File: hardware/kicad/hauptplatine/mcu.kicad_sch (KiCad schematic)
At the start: 31 parts, among them J301 USB-C, J302 Debug (SWD + Serial1), SW301 Reset, SW302 BOOT, SW303 Service, SW304 Reedkontakt, U301 STM32F411CEU6, U302 USBLC6-2SC6, Y301 25MHz 12pF, Y302 32,768k 7pF

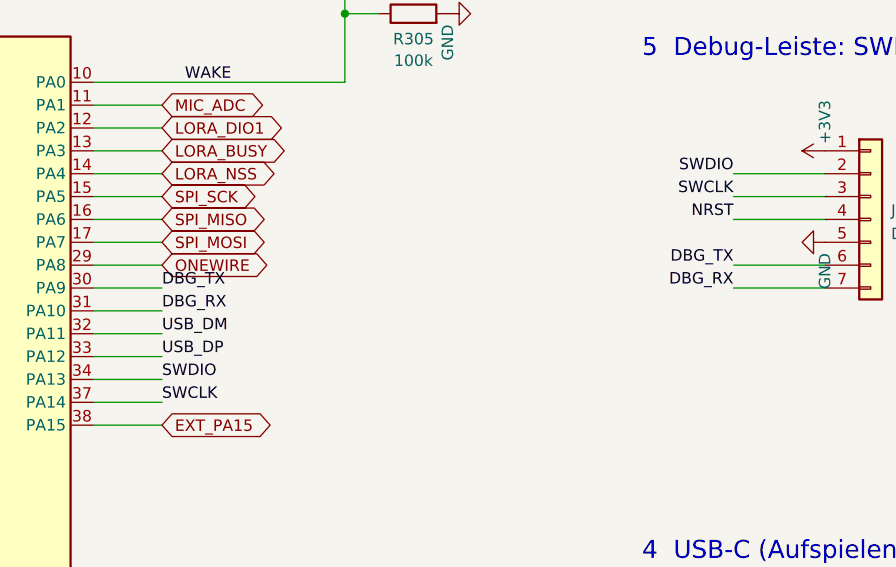
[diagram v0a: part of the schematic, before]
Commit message: update
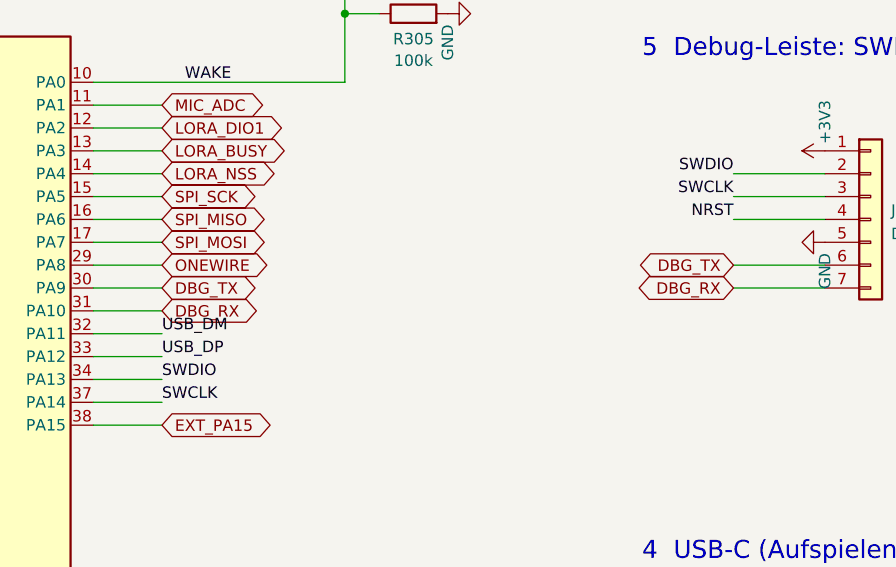
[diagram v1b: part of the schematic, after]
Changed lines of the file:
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@@
-		)
-	)
-	(label "DBG_TX"
-		(at 289.56 124.46 180)
-		(effects
-			(font
-				(size 1.27 1.27)
-			)
-			(justify right bottom)
 		)
 	)
@@
 		)
 	)
-	(label "DBG_TX"
-		(at 226.06 127 0)
-		(effects
-			(font
-				(size 1.27 1.27)
-			)
-			(justify left bottom)
-		)
-	)
 	(label "USB_CC1"
 		(at 292.1 214.63 90)
@@
 		)
 	)
-	(label "DBG_RX"
-		(at 226.06 129.54 0)
-		(effects
-			(font
-				(size 1.27 1.27)
-			)
-			(justify left bottom)
-		)
-	)
 	(label "VDDA"
 		(at 207.01 81.28 0)
@@
 		)
 	)
-	(label "DBG_RX"
-		(at 289.56 127 180)
-		(effects
-			(font
-				(size 1.27 1.27)
-			)
-			(justify right bottom)
-		)
-	)
 	(label "BOOT1"
 		(at 86.36 151.13 90)
@@
 		)
 	)
+	(global_label "DBG_TX"
+		(shape bidirectional)
+		(at 289.56 124.46 180)
+		(fields_autoplaced yes)
+		(effects
+			(font
+				(size 1.27 1.27)
+			)
+			(justify right)
+		)
+		(property "Intersheetrefs" "${INTERSHEET_REFS}"
+			(at 289.56 124.46 0)
+			(hide yes)
+			(show_name no)
+			(do_not_autoplace no)
+			(effects
+				(font
+					(size 1.27 1.27)
+				)
+			)
+		)
+	)
 	(global_label "LORA_NSS"
 		(shape bidirectional)
@@
 		)
 	)
+	(global_label "DBG_TX"
+		(shape bidirectional)
+		(at 226.06 127 0)
+		(fields_autoplaced yes)
+		(effects
+			(font
+				(size 1.27 1.27)
+			)
+			(justify left)
+		)
+		(property "Intersheetrefs" "${INTERSHEET_REFS}"
+			(at 226.06 127 0)
+			(hide yes)
+			(show_name no)
+			(do_not_autoplace no)
+			(effects
+				(font
+					(size 1.27 1.27)
+				)
+			)
+		)
+	)
 	(global_label "MIC_ADC"
 		(shape bidirectional)
@@
 		)
 	)
+	(global_label "DBG_RX"
+		(shape bidirectional)
+		(at 226.06 129.54 0)
+		(fields_autoplaced yes)
+		(effects
+			(font
+				(size 1.27 1.27)
+			)
+			(justify left)
+		)
+		(property "Intersheetrefs" "${INTERSHEET_REFS}"
+			(at 226.06 129.54 0)
+			(hide yes)
+			(show_name no)
+			(do_not_autoplace no)
+			(effects
+				(font
+					(size 1.27 1.27)
+				)
+			)
+		)
+	)
 	(global_label "EXT_PB13"
 		(shape bidirectional)
@@
 			(hide yes)
 			(show_name no)
+			(do_not_autoplace no)
+			(effects
+				(font
+					(size 1.27 1.27)
+				)
+			)
+		)
+	)
+	(global_label "DBG_RX"
+		(shape bidirectional)
+		(at 289.56 127 180)
+		(fields_autoplaced yes)
+		(effects
+			(font
+				(size 1.27 1.27)
+			)
+			(justify right)
+		)
+		(property "Intersheetrefs" "${INTERSHEET_REFS}"
+			(at 289.56 127 0)
+			(hide yes)
+			(show_name no)
